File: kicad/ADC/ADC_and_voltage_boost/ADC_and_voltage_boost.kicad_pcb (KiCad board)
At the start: 2 copper layers, 32.5 x 42 mm, 13 parts, among them J1 Screw_Terminal_01x04, J2 Screw_Terminal_01x04, J3 Screw_Terminal_01x02, U3 MOUDLE-SEEEDUINO-XIAO-ESP32C3, U4 MAX1032BEUG_

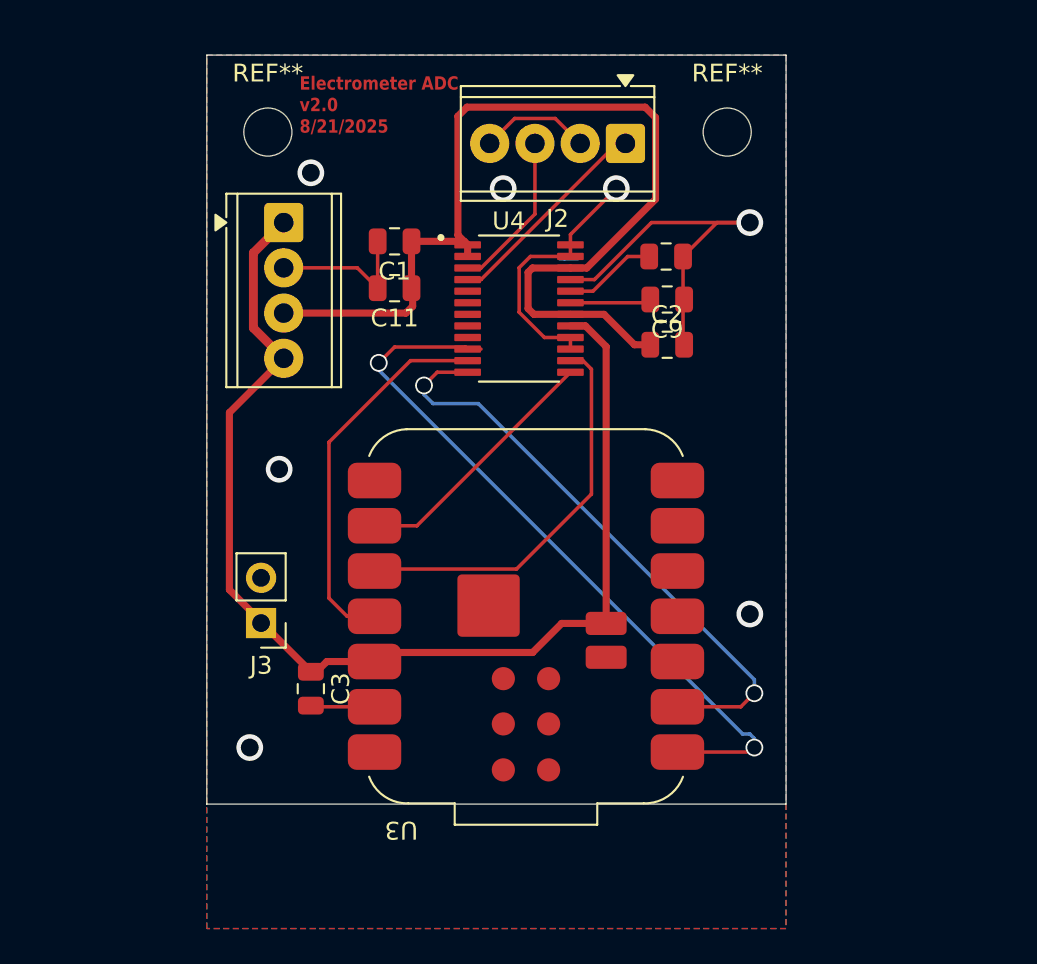
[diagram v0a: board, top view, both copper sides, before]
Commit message: fixing board issues - kicad
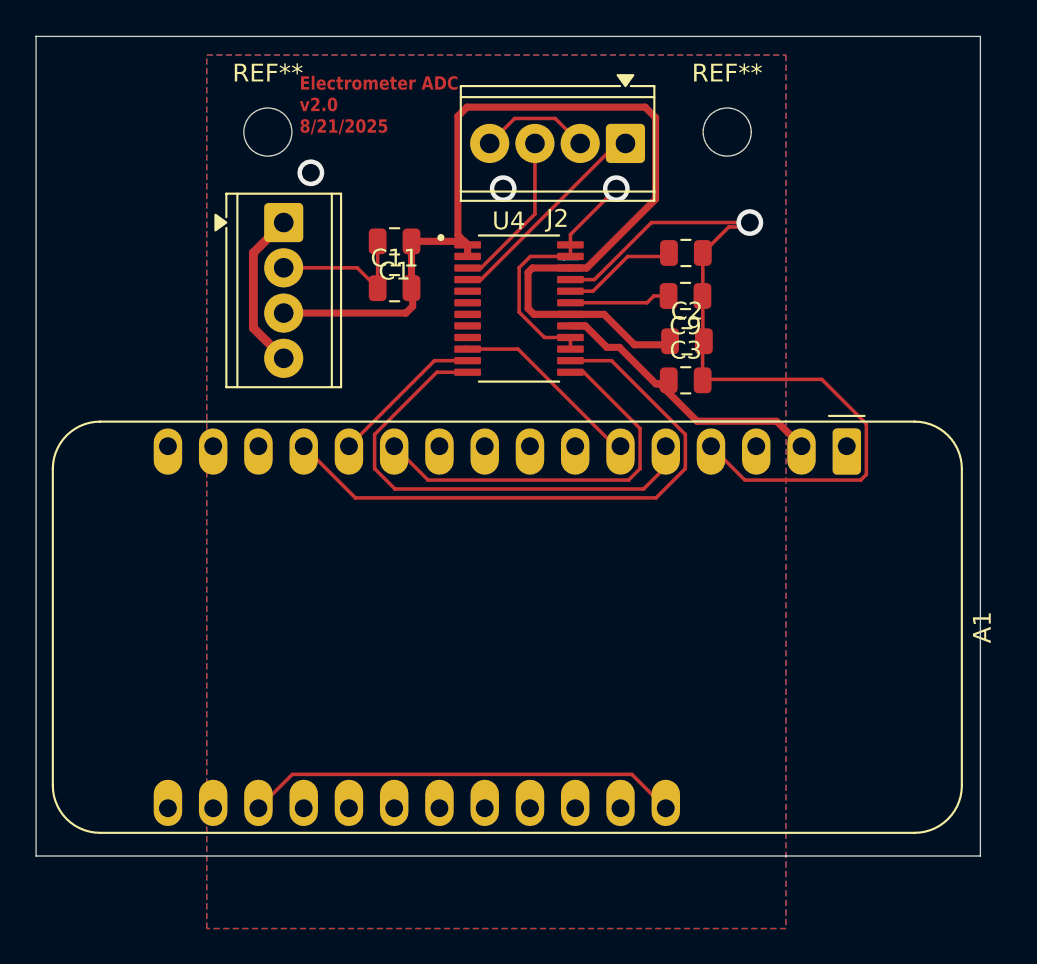
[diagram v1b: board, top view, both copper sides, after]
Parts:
- removed J3: Screw_Terminal_01x02, Connector_PinHeader_2.54mm:PinHeader_1x02_P2.54mm_Vertical
- removed U3: MOUDLE-SEEEDUINO-XIAO-ESP32C3, RF_Module:MCU_Seeed_ESP32C3
- added A1: Adafruit_Feather_HUZZAH32_ESP32, Module:Adafruit_Feather, F.Cu at (168.0, 104.5)
- moved C3 27.2 mm to (159.0, 100.8), turned to 0 degrees
- moved C2 1.13 mm to (159.0, 98.6)
- moved C8 1.13 mm to (159.0, 93.7)
- moved C9 1.05 mm to (158.9, 96.1)
- turned C11 to 0 degrees
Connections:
- C11 pad 1: +5V -> GND
- C11 pad 2: GND -> +5V
- U4 pad 12: Net-(U3-PA4_A1_D1) -> /SSTRB
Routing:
- net +BATT: track 65.5 -> 25.4 mm
- net Net-(U3-PA4_A1_D1): track 33.8 -> 0.00 mm, vias 2 -> 0
- net /~{CS}: track 41.1 -> 11.0 mm, vias 2 -> 0
- net /SSTRB: track 0.00 -> 27.1 mm
- net Net-(A1-A6/IO14): track 0.00 -> 24.4 mm
- net GND: track 54.6 -> 75.1 mm, vias 7 -> 4
- net /MOSI: track 21.4 -> 8.65 mm
- net /MISO: track 22.4 -> 33.4 mm
- net /SCK: track 14.6 -> 22.3 mm
- net Net-(U4-REFCAP): track 4.56 -> 5.95 mm
- net Net-(U4-REF): track 5.23 -> 6.42 mm
- net +5V: track 57.1 -> 58.3 mm
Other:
- board size 32.5 x 42 mm -> 53 x 46 mm
